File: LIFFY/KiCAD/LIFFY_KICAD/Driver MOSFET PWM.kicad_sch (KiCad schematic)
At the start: 15 parts, among them J13 LEDBAR2, J7 LEDBAR1, Q1 IRF3205, Q2 IRF3205, U4 MIC4427

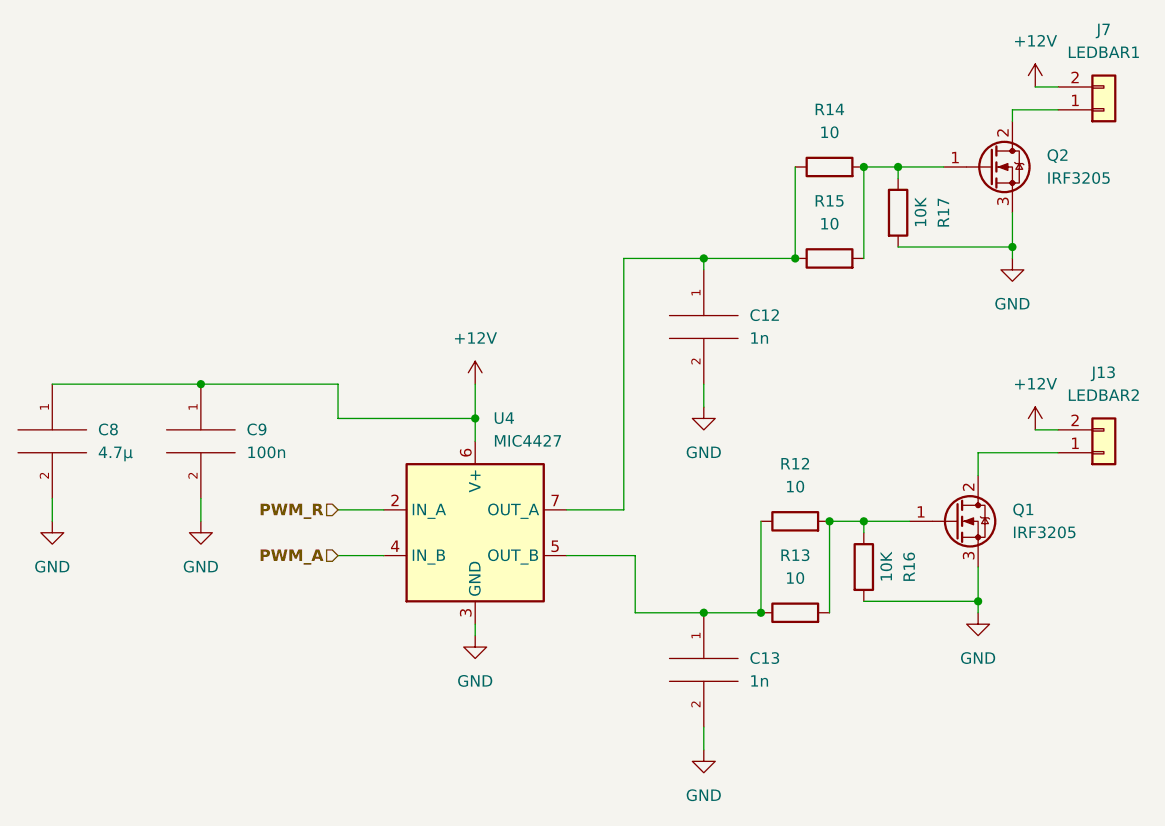
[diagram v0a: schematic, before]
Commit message: V4.5 Fixed
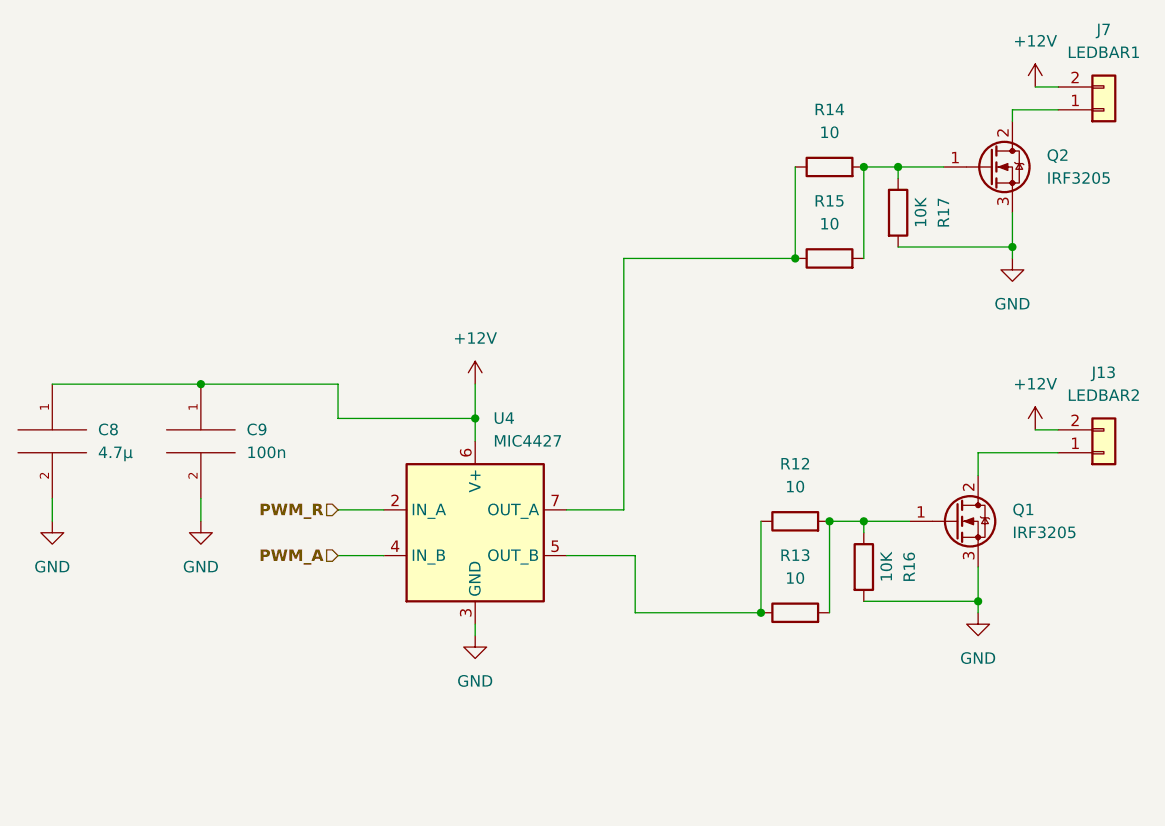
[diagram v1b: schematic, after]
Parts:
- removed C12, C13: 1n, Capacitor_SMD:C_0201_0603Metric, symbol pspice:CAP
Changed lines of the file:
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@@
   (junction (at 181.61 110.49) (diameter 0) (color 0 0 0 0)
   )
-  (junction (at 151.13 111.76) (diameter 0) (color 0 0 0 0)
-  )
   (junction (at 157.48 111.76) (diameter 0) (color 0 0 0 0)
   )
   (junction (at 185.42 71.12) (diameter 0) (color 0 0 0 0)
   )
-  (junction (at 151.13 72.39) (diameter 0) (color 0 0 0 0)
-  )
   (junction (at 125.73 90.17) (diameter 0) (color 0 0 0 0)
   )
@@
     (stroke (width 0) (type default) (color 0 0 0 0))
   )
-  (wire (pts (xy 151.13 72.39) (xy 151.13 73.66))
-    (stroke (width 0) (type default) (color 0 0 0 0))
-  )
   (wire (pts (xy 168.91 110.49) (xy 181.61 110.49))
     (stroke (width 0) (type default) (color 0 0 0 0))
@@
     (stroke (width 0) (type default) (color 0 0 0 0))
   )
-  (wire (pts (xy 151.13 111.76) (xy 157.48 111.76))
-    (stroke (width 0) (type default) (color 0 0 0 0))
-  )
   (wire (pts (xy 125.73 86.36) (xy 125.73 90.17))
     (stroke (width 0) (type default) (color 0 0 0 0))
   )
-  (wire (pts (xy 151.13 86.36) (xy 151.13 88.9))
-    (stroke (width 0) (type default) (color 0 0 0 0))
-  )
-  (wire (pts (xy 143.51 111.76) (xy 151.13 111.76))
+  (wire (pts (xy 143.51 111.76) (xy 157.48 111.76))
     (stroke (width 0) (type default) (color 0 0 0 0))
   )
@@
     (stroke (width 0) (type default) (color 0 0 0 0))
   )
-  (wire (pts (xy 151.13 72.39) (xy 161.29 72.39))
-    (stroke (width 0) (type default) (color 0 0 0 0))
-  )
   (wire (pts (xy 187.96 53.34) (xy 190.5 53.34))
     (stroke (width 0) (type default) (color 0 0 0 0))
   )
-  (wire (pts (xy 151.13 124.46) (xy 151.13 127))
-    (stroke (width 0) (type default) (color 0 0 0 0))
-  )
   (wire (pts (xy 168.91 101.6) (xy 173.99 101.6))
     (stroke (width 0) (type default) (color 0 0 0 0))
@@
     (stroke (width 0) (type default) (color 0 0 0 0))
   )
-  (wire (pts (xy 142.24 72.39) (xy 151.13 72.39))
+  (wire (pts (xy 142.24 72.39) (xy 161.29 72.39))
     (stroke (width 0) (type default) (color 0 0 0 0))
   )
@@
     (pin "2")
   )
-  (symbol (lib_id "pspice:CAP") (at 151.13 118.11 0) (unit 1)
-    (in_bom yes) (on_board yes) (fields_autoplaced)
-    (property "Reference" "C13" (id 0) (at 156.21 116.8399 0)
-      (effects (font (size 1.27 1.27)) (justify left))
-    )
-    (property "Value" "1n" (id 1) (at 156.21 119.3799 0)
-      (effects (font (size 1.27 1.27)) (justify left))
-    )
-    (property "Footprint" "Capacitor_SMD:C_0201_0603Metric" (id 2) (at 151.13 118.11 0)
-      (effects (font (size 1.27 1.27)) hide)
-    )
-    (property "Datasheet" "~" (id 3) (at 151.13 118.11 0)
-      (effects (font (size 1.27 1.27)) hide)
-    )
-    (pin "1")
-    (pin "2")
-  )
   (symbol (lib_id "power:GND") (at 95.25 101.6 0) (unit 1)
     (in_bom yes) (on_board yes)
@@
     (pin "2")
   )
-  (symbol (lib_id "power:GND") (at 151.13 127 0) (unit 1)
-    (in_bom yes) (on_board yes)
-    (property "Reference" "#PWR0120" (id 0) (at 151.13 133.35 0)
-      (effects (font (size 1.27 1.27)) hide)
-    )
-    (property "Value" "GND" (id 1) (at 151.13 132.08 0))
-    (property "Footprint" "" (id 2) (at 151.13 127 0)
-      (effects (font (size 1.27 1.27)) hide)
-    )
-    (property "Datasheet" "" (id 3) (at 151.13 127 0)
-      (effects (font (size 1.27 1.27)) hide)
-    )
-    (pin "1")
-  )
   (symbol (lib_id "power:+12V") (at 125.73 86.36 0) (unit 1)
     (in_bom yes) (on_board yes) (fields_autoplaced)
@@
     )
     (pin "1")
-  )
-  (symbol (lib_id "pspice:CAP") (at 151.13 80.01 0) (unit 1)
-    (in_bom yes) (on_board yes) (fields_autoplaced)
-    (property "Reference" "C12" (id 0) (at 156.21 78.7399 0)
-      (effects (font (size 1.27 1.27)) (justify left))
-    )
-    (property "Value" "1n" (id 1) (at 156.21 81.2799 0)
-      (effects (font (size 1.27 1.27)) (justify left))
-    )
-    (property "Footprint" "Capacitor_SMD:C_0201_0603Metric" (id 2) (at 151.13 80.01 0)
-      (effects (font (size 1.27 1.27)) hide)
-    )
-    (property "Datasheet" "~" (id 3) (at 151.13 80.01 0)
-      (effects (font (size 1.27 1.27)) hide)
-    )
-    (pin "1")
-    (pin "2")
   )
   (symbol (lib_id "power:+12V") (at 187.96 91.44 0) (unit 1)
@@
     (pin "2")
   )
-  (symbol (lib_id "power:GND") (at 151.13 88.9 0) (unit 1)
-    (in_bom yes) (on_board yes)
-    (property "Reference" "#PWR0121" (id 0) (at 151.13 95.25 0)
-      (effects (font (size 1.27 1.27)) hide)
-    )
-    (property "Value" "GND" (id 1) (at 151.13 93.98 0))
-    (property "Footprint" "" (id 2) (at 151.13 88.9 0)
-      (effects (font (size 1.27 1.27)) hide)
-    )
-    (property "Datasheet" "" (id 3) (at 151.13 88.9 0)
-      (effects (font (size 1.27 1.27)) hide)
-    )
-    (pin "1")
-  )
   (symbol (lib_id "Device:R") (at 172.72 67.31 0) (unit 1)

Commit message: V3 Fixed
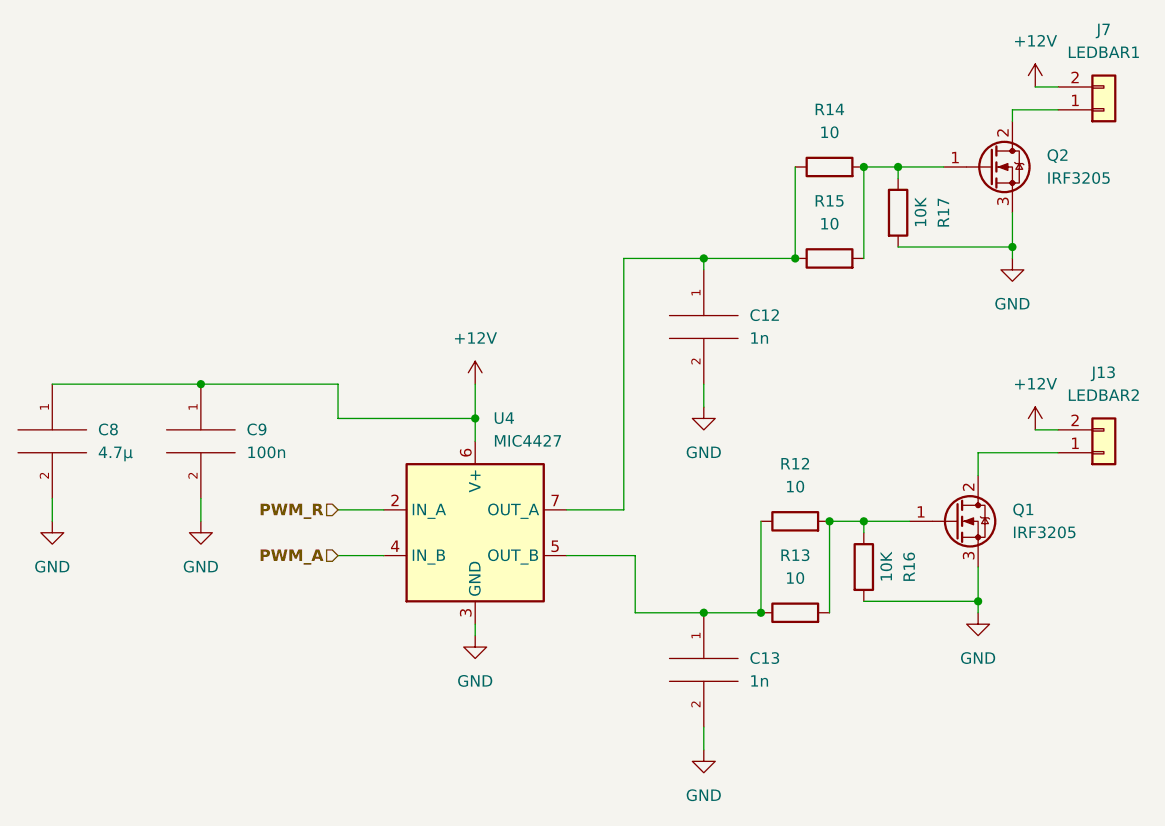
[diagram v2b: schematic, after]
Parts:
- added C12, C13: 1n, Capacitor_SMD:C_0201_0603Metric, symbol pspice:CAP
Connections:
- net GND: now also C12.2, C13.2
- net at R12.1, R13.1, U4.5 (OUT_B): now also C13.1
- net at R14.1, R15.1, U4.7 (OUT_A): now also C12.1
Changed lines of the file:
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@@
   (junction (at 181.61 110.49) (diameter 0) (color 0 0 0 0)
   )
+  (junction (at 151.13 111.76) (diameter 0) (color 0 0 0 0)
+  )
   (junction (at 157.48 111.76) (diameter 0) (color 0 0 0 0)
   )
   (junction (at 185.42 71.12) (diameter 0) (color 0 0 0 0)
   )
+  (junction (at 151.13 72.39) (diameter 0) (color 0 0 0 0)
+  )
   (junction (at 125.73 90.17) (diameter 0) (color 0 0 0 0)
   )
@@
     (stroke (width 0) (type default) (color 0 0 0 0))
   )
+  (wire (pts (xy 151.13 72.39) (xy 151.13 73.66))
+    (stroke (width 0) (type default) (color 0 0 0 0))
+  )
   (wire (pts (xy 168.91 110.49) (xy 181.61 110.49))
     (stroke (width 0) (type default) (color 0 0 0 0))
@@
     (stroke (width 0) (type default) (color 0 0 0 0))
   )
+  (wire (pts (xy 151.13 111.76) (xy 157.48 111.76))
+    (stroke (width 0) (type default) (color 0 0 0 0))
+  )
   (wire (pts (xy 125.73 86.36) (xy 125.73 90.17))
     (stroke (width 0) (type default) (color 0 0 0 0))
   )
-  (wire (pts (xy 143.51 111.76) (xy 157.48 111.76))
+  (wire (pts (xy 151.13 86.36) (xy 151.13 88.9))
+    (stroke (width 0) (type default) (color 0 0 0 0))
+  )
+  (wire (pts (xy 143.51 111.76) (xy 151.13 111.76))
     (stroke (width 0) (type default) (color 0 0 0 0))
   )
@@
     (stroke (width 0) (type default) (color 0 0 0 0))
   )
+  (wire (pts (xy 151.13 72.39) (xy 161.29 72.39))
+    (stroke (width 0) (type default) (color 0 0 0 0))
+  )
   (wire (pts (xy 187.96 53.34) (xy 190.5 53.34))
     (stroke (width 0) (type default) (color 0 0 0 0))
   )
+  (wire (pts (xy 151.13 124.46) (xy 151.13 127))
+    (stroke (width 0) (type default) (color 0 0 0 0))
+  )
   (wire (pts (xy 168.91 101.6) (xy 173.99 101.6))
     (stroke (width 0) (type default) (color 0 0 0 0))
@@
     (stroke (width 0) (type default) (color 0 0 0 0))
   )
-  (wire (pts (xy 142.24 72.39) (xy 161.29 72.39))
+  (wire (pts (xy 142.24 72.39) (xy 151.13 72.39))
     (stroke (width 0) (type default) (color 0 0 0 0))
   )
@@
     (pin "2")
   )
+  (symbol (lib_id "pspice:CAP") (at 151.13 118.11 0) (unit 1)
+    (in_bom yes) (on_board yes) (fields_autoplaced)
+    (property "Reference" "C13" (id 0) (at 156.21 116.8399 0)
+      (effects (font (size 1.27 1.27)) (justify left))
+    )
+    (property "Value" "1n" (id 1) (at 156.21 119.3799 0)
+      (effects (font (size 1.27 1.27)) (justify left))
+    )
+    (property "Footprint" "Capacitor_SMD:C_0201_0603Metric" (id 2) (at 151.13 118.11 0)
+      (effects (font (size 1.27 1.27)) hide)
+    )
+    (property "Datasheet" "~" (id 3) (at 151.13 118.11 0)
+      (effects (font (size 1.27 1.27)) hide)
+    )
+    (pin "1")
+    (pin "2")
+  )
   (symbol (lib_id "power:GND") (at 95.25 101.6 0) (unit 1)
     (in_bom yes) (on_board yes)
@@
     (pin "2")
   )
+  (symbol (lib_id "power:GND") (at 151.13 127 0) (unit 1)
+    (in_bom yes) (on_board yes)
+    (property "Reference" "#PWR0120" (id 0) (at 151.13 133.35 0)
+      (effects (font (size 1.27 1.27)) hide)
+    )
+    (property "Value" "GND" (id 1) (at 151.13 132.08 0))
+    (property "Footprint" "" (id 2) (at 151.13 127 0)
+      (effects (font (size 1.27 1.27)) hide)
+    )
+    (property "Datasheet" "" (id 3) (at 151.13 127 0)
+      (effects (font (size 1.27 1.27)) hide)
+    )
+    (pin "1")
+  )
   (symbol (lib_id "power:+12V") (at 125.73 86.36 0) (unit 1)
     (in_bom yes) (on_board yes) (fields_autoplaced)
@@
     )
     (pin "1")
+  )
+  (symbol (lib_id "pspice:CAP") (at 151.13 80.01 0) (unit 1)
+    (in_bom yes) (on_board yes) (fields_autoplaced)
+    (property "Reference" "C12" (id 0) (at 156.21 78.7399 0)
+      (effects (font (size 1.27 1.27)) (justify left))
+    )
+    (property "Value" "1n" (id 1) (at 156.21 81.2799 0)
+      (effects (font (size 1.27 1.27)) (justify left))
+    )
+    (property "Footprint" "Capacitor_SMD:C_0201_0603Metric" (id 2) (at 151.13 80.01 0)
+      (effects (font (size 1.27 1.27)) hide)
+    )
+    (property "Datasheet" "~" (id 3) (at 151.13 80.01 0)
+      (effects (font (size 1.27 1.27)) hide)
+    )
+    (pin "1")
+    (pin "2")
   )
   (symbol (lib_id "power:+12V") (at 187.96 91.44 0) (unit 1)
@@
     (pin "2")
   )
+  (symbol (lib_id "power:GND") (at 151.13 88.9 0) (unit 1)
+    (in_bom yes) (on_board yes)
+    (property "Reference" "#PWR0121" (id 0) (at 151.13 95.25 0)
+      (effects (font (size 1.27 1.27)) hide)
+    )
+    (property "Value" "GND" (id 1) (at 151.13 93.98 0))
+    (property "Footprint" "" (id 2) (at 151.13 88.9 0)
+      (effects (font (size 1.27 1.27)) hide)
+    )
+    (property "Datasheet" "" (id 3) (at 151.13 88.9 0)
+      (effects (font (size 1.27 1.27)) hide)
+    )
+    (pin "1")
+  )
   (symbol (lib_id "Device:R") (at 172.72 67.31 0) (unit 1)
